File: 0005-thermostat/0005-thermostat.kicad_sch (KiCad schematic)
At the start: 20 parts, among them J1 NTC2, J3 12V, P1 22k, P2 22k

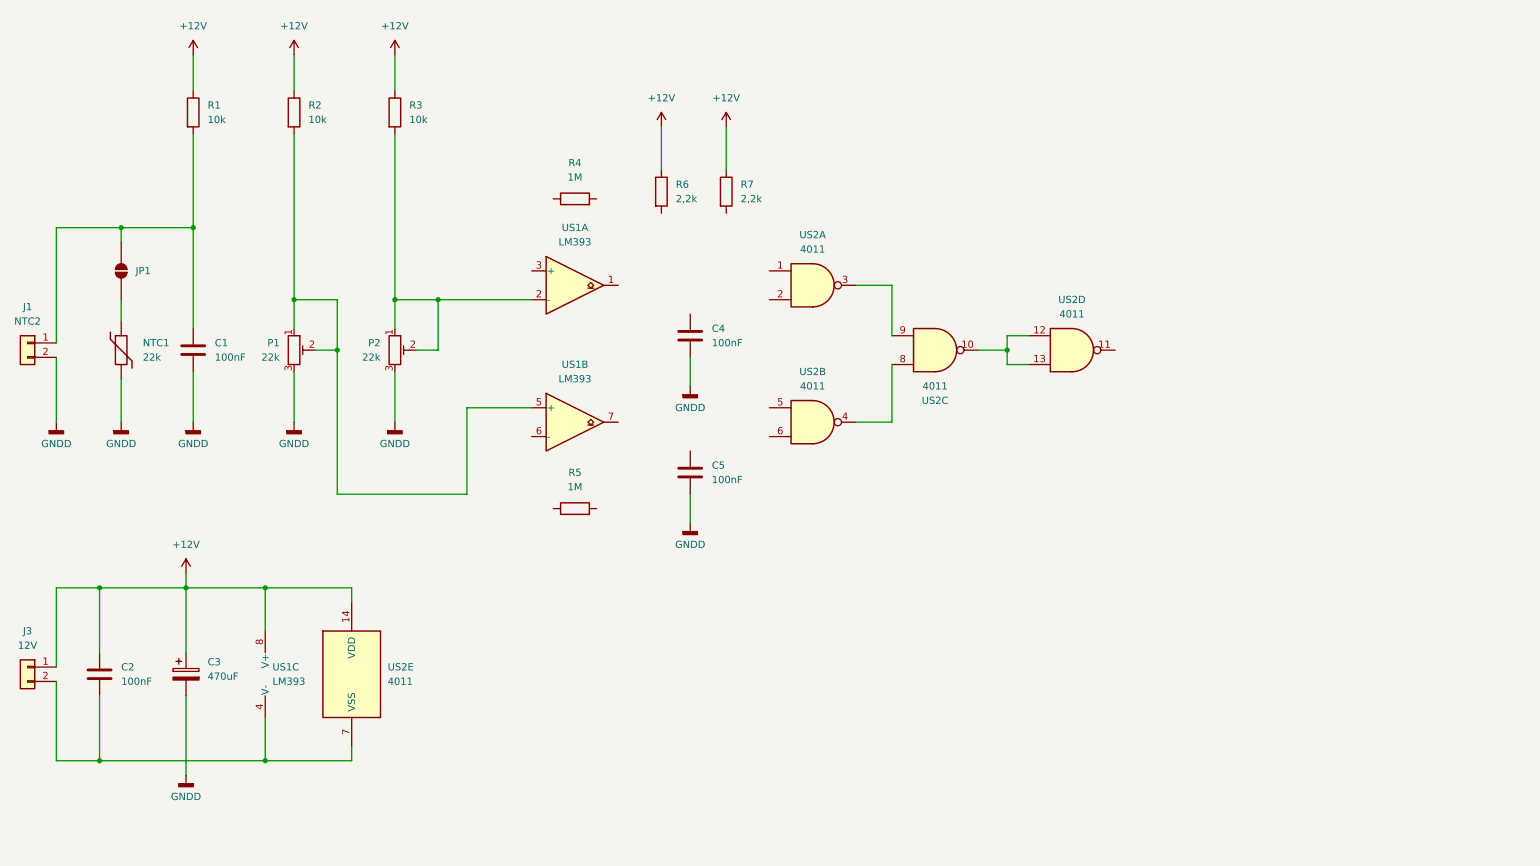
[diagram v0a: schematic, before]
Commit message: Schematic complete
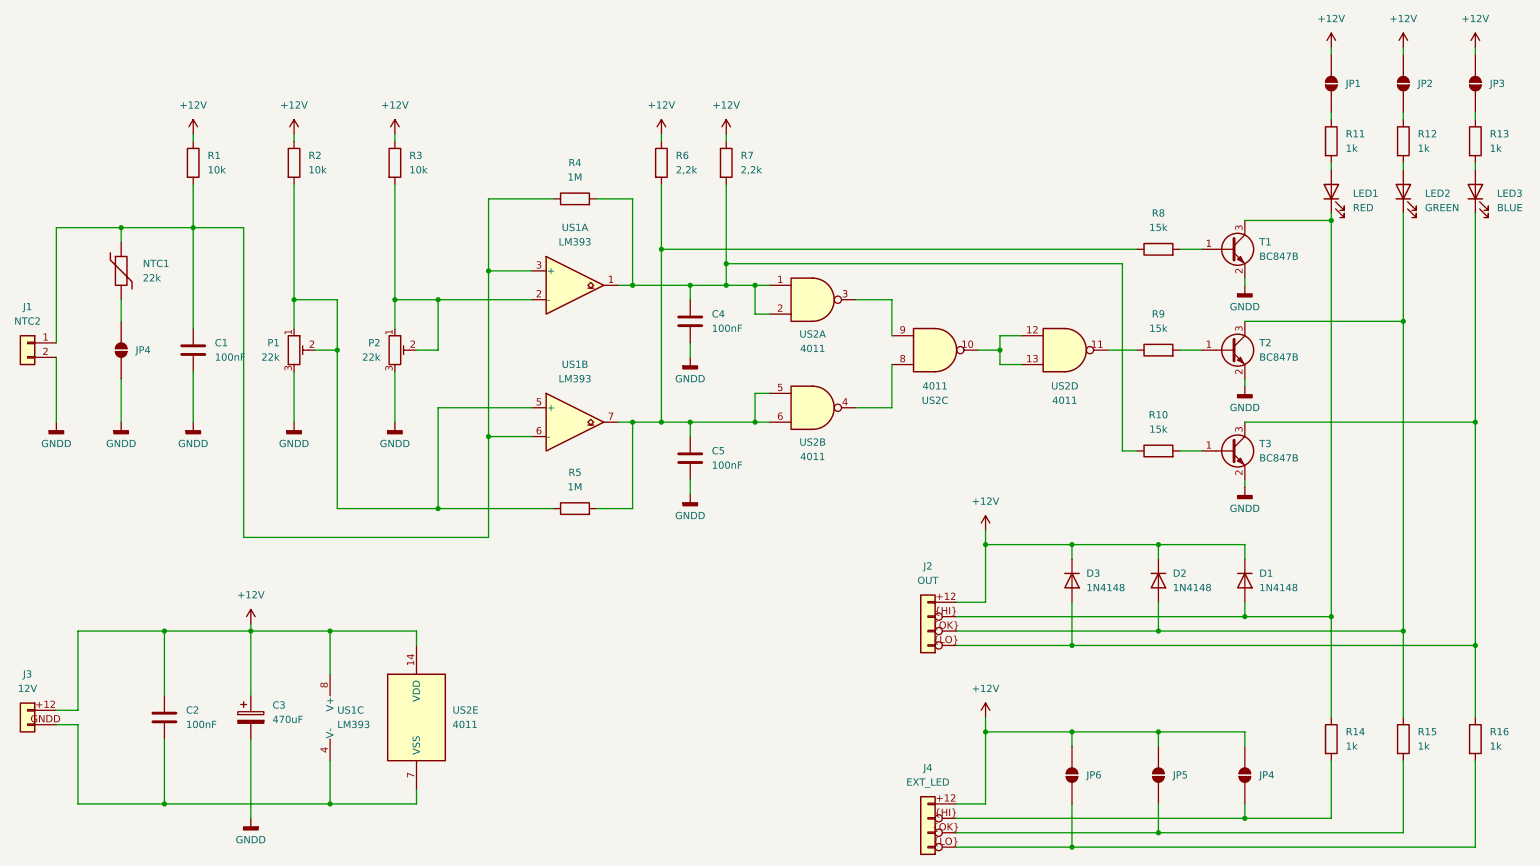
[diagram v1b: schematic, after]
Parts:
- added D1, D2, D3: 1N4148, Diode_THT:D_DO-35_SOD27_P7.62mm_Horizontal, symbol Diode:1N4148
- added J2: OUT, symbol Connector_Generic:Conn_01x04
- added J4: EXT_LED, symbol Connector_Generic:Conn_01x04
- added JP1, JP2, JP3, JP4, JP5, JP6: SolderJumper_2_Open, symbol Jumper:SolderJumper_2_Open
- added LED1: RED, symbol Device:LED
- added LED2: GREEN, symbol Device:LED
- added LED3: BLUE, symbol Device:LED
- added R10, R8, R9: 15k, symbol Device:R
- added R11, R12, R13, R14, R15, R16: 1k, symbol Device:R
- added T1, T2, T3: BC847B, Package_TO_SOT_SMD:SOT-23, symbol Transistor_BJT:BC847
- renumbered JP1 to JP4
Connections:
- net +12V: now also J3.+12 (Pin_1), D1.1 (K), D2.1 (K), D3.1 (K), J2.+12 (Pin_4), J4.+12 (Pin_4), JP1.2 (B), JP2.2 (B), JP3.2 (B), JP4.2 (B), JP5.2 (B), JP6.2 (B); no longer J3.1 (Pin_1)
- net GNDD: now also JP4.1 (A), T1.2 (E), T2.2 (E), T3.2 (E); no longer NTC1.2
- net at C4.1: now also R4.2, R7.2, US1.1, US2.1, US2.2, R10.1
- net at P1.1, P1.2, R2.2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: now also R5.1
- net at US2.5: now also C5.1, R5.2, R6.2, US1.7, US2.6, R8.1
- net at C2.2, US1.4 (V-), US2.7 (VSS): now also J3.GNDD (Pin_2); no longer J3.2 (Pin_2)
- net at US1.6 (-): now also C1.1, J1.1 (Pin_1), NTC1.1, R1.2, R4.1, US1.3 (+)
- net at US2.11: now also R9.1
- new net: R8.2, T1.1 (B)
- new net: D1.2 (A), J2.~{HI} (Pin_3), LED1.1 (K), R14.1, T1.3 (C)
- new net: D3.2 (A), J2.~{LO} (Pin_1), LED3.1 (K), R16.1, T3.3 (C)
- new net: D2.2 (A), J2.~{OK} (Pin_2), LED2.1 (K), R15.1, T2.3 (C)
- new net: JP2.1 (A), R12.1
- new net: LED3.2 (A), R13.2
- new net: JP3.1 (A), R13.1
- new net: R10.2, T3.1 (B)
- new net: LED2.2 (A), R12.2
- new net: J4.~{OK} (Pin_2), JP5.1 (A), R15.2
- new net: J4.~{HI} (Pin_3), JP4.1 (A), R14.2
- new net: J4.~{LO} (Pin_1), JP6.1 (A), R16.2
- new net: JP1.1 (A), R11.1
- new net: R9.2, T2.1 (B)
- new net: LED1.2 (A), R11.2
- new net: JP4.2 (B), NTC1.2
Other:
- moved on the sheet: C2, C3, C4, C5, J3, JP4, NTC1, R1, R2, R3, R6, R7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
